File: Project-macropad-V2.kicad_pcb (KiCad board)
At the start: 2 copper layers, 110.5 x 128.4 mm, 51 parts, among them J1 Conn_01x04_Male, SW1 RotaryEncoder_Switch, SW2 SW_Push, SW3 SW_SPDT

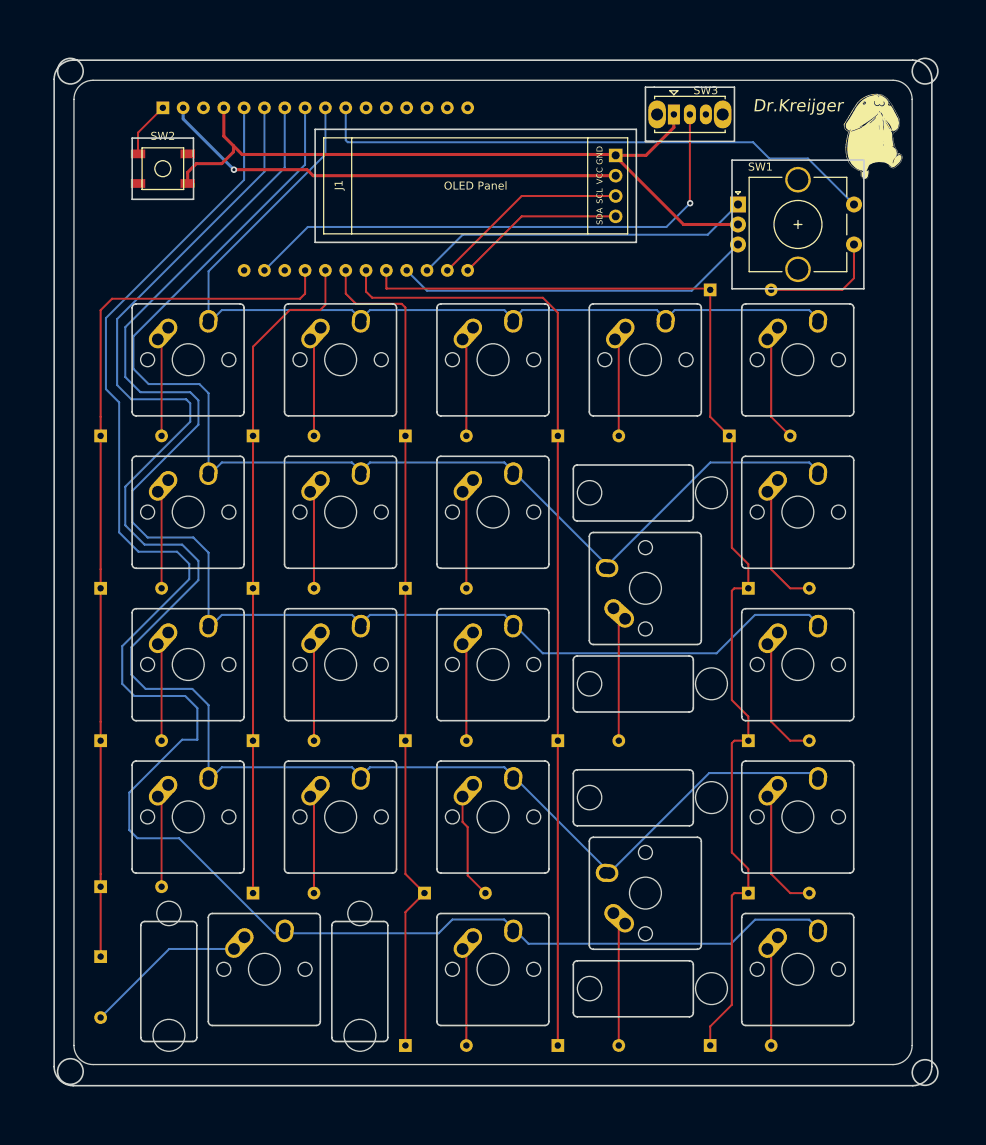
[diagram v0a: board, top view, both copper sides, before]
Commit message: Plate done
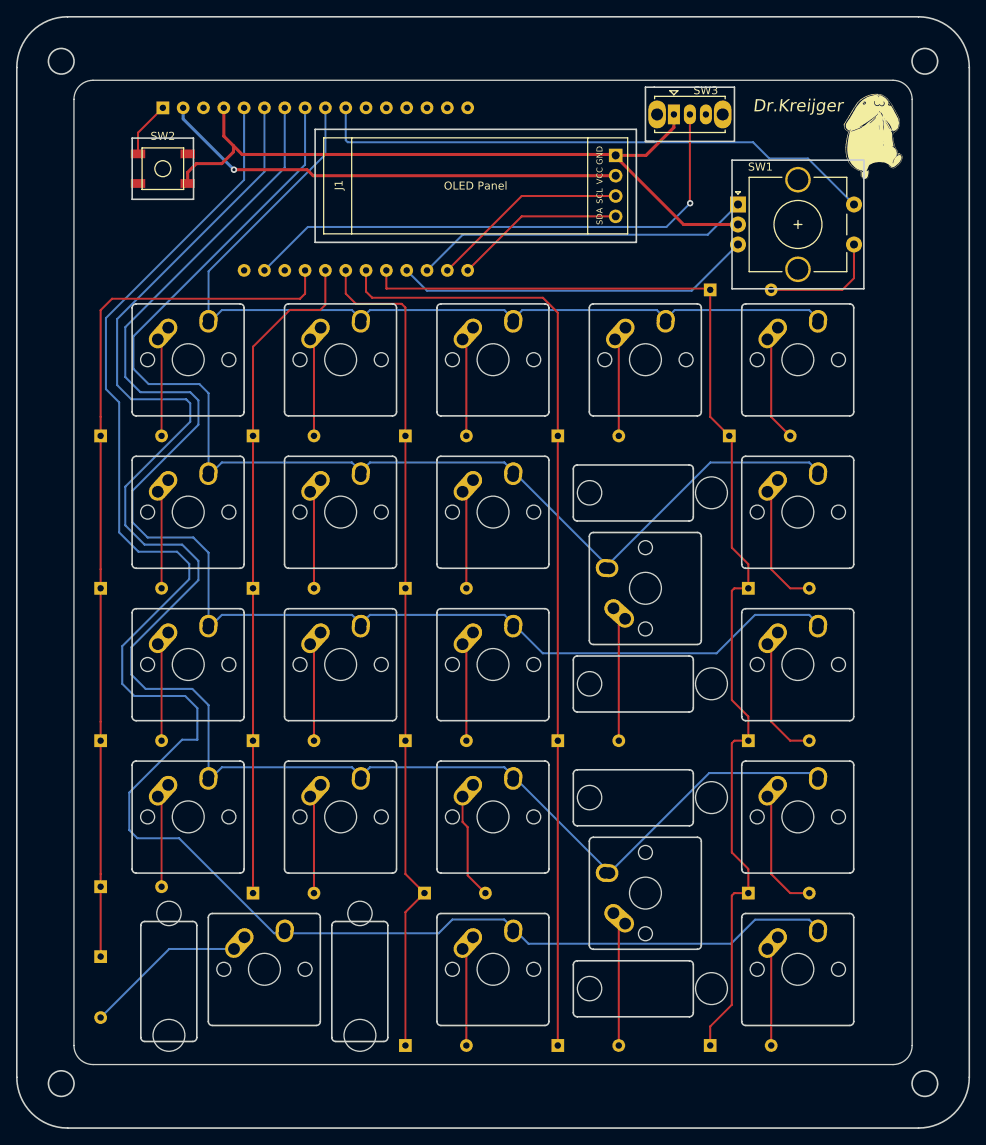
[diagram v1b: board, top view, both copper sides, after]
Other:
- board size 110.5 x 128.4 mm -> 119.1 x 138.9 mm
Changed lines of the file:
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@@
   (gr_line (start 113.635 50.673) (end 113.635 63.673) (layer "Edge.Cuts") (width 0.2))
   (gr_line (start 203.835 88.773) (end 203.835 101.773) (layer "Edge.Cuts") (width 0.2))
-  (gr_line (start 106.26725 147.898) (end 211.219002 147.898) (layer "Edge.Cuts") (width 0.2))
-  (gr_circle (center 105.918 21.082) (end 107.518 21.082) (layer "Edge.Cuts") (width 0.2) (fill none))
+  (gr_circle (center 104.775 19.84375) (end 106.375 19.84375) (layer "Edge.Cuts") (width 0.2) (fill none))
   (gr_arc (start 189.835 126.873) (mid 189.981447 126.519447) (end 190.335 126.373) (layer "Edge.Cuts") (width 0.2))
   (gr_arc (start 152.235 83.223) (mid 151.881447 83.076553) (end 151.735 82.723) (layer "Edge.Cuts") (width 0.2))
@@
   (gr_arc (start 127.135 88.273) (mid 127.488553 88.419447) (end 127.635 88.773) (layer "Edge.Cuts") (width 0.2))
   (gr_line (start 132.685 69.723) (end 132.685 82.723) (layer "Edge.Cuts") (width 0.2))
+  (gr_arc (start 211.93125 14.2875) (mid 216.421378 16.147372) (end 218.28125 20.6375) (layer "Edge.Cuts") (width 0.2))
   (gr_line (start 132.685 50.673) (end 132.685 63.673) (layer "Edge.Cuts") (width 0.2))
   (gr_line (start 132.685 107.823) (end 132.685 120.823) (layer "Edge.Cuts") (width 0.2))
   (gr_arc (start 170.785 79.248) (mid 170.931447 78.894447) (end 171.285 78.748) (layer "Edge.Cuts") (width 0.2))
+  (gr_line (start 99.21875 20.6375) (end 99.21875 146.84375) (layer "Edge.Cuts") (width 0.2))
   (gr_arc (start 113.635 107.823) (mid 113.781447 107.469447) (end 114.135 107.323) (layer "Edge.Cuts") (width 0.2))
   (gr_line (start 113.6396 29.448) (end 113.6396 37.084) (layer "Edge.Cuts") (width 0.2))
@@
   (gr_arc (start 127.635 63.673) (mid 127.488553 64.026553) (end 127.135 64.173) (layer "Edge.Cuts") (width 0.2))
   (gr_arc (start 123.16 126.873) (mid 123.306447 126.519447) (end 123.66 126.373) (layer "Edge.Cuts") (width 0.2))
-  (gr_circle (center 212.7506 21.082) (end 214.3506 21.082) (layer "Edge.Cuts") (width 0.2) (fill none))
+  (gr_circle (center 212.725 19.84375) (end 214.325 19.84375) (layer "Edge.Cuts") (width 0.2) (fill none))
   (gr_line (start 152.235 121.323) (end 165.235 121.323) (layer "Edge.Cuts") (width 0.2))
   (gr_arc (start 203.335 50.173) (mid 203.688553 50.319447) (end 203.835 50.673) (layer "Edge.Cuts") (width 0.2))
@@
   (gr_arc (start 127.135 50.173) (mid 127.488553 50.319447) (end 127.635 50.673) (layer "Edge.Cuts") (width 0.2))
   (gr_line (start 114.135 107.323) (end 127.135 107.323) (layer "Edge.Cuts") (width 0.2))
-  (gr_line (start 213.600252 145.51675) (end 213.600252 22.09165) (layer "Edge.Cuts") (width 0.2))
-  (gr_arc (start 213.600252 145.51675) (mid 212.9028 147.200548) (end 211.219002 147.898) (layer "Edge.Cuts") (width 0.2))
   (gr_line (start 170.785 79.248) (end 170.785 92.248) (layer "Edge.Cuts") (width 0.2))
   (gr_arc (start 189.835 50.673) (mid 189.981447 50.319447) (end 190.335 50.173) (layer "Edge.Cuts") (width 0.2))
@@
   (gr_line (start 170.785 50.673) (end 170.785 63.673) (layer "Edge.Cuts") (width 0.2))
   (gr_arc (start 183.285 108.41) (mid 183.638553 108.556447) (end 183.785 108.91) (layer "Edge.Cuts") (width 0.2))
-  (gr_line (start 211.219002 19.7104) (end 106.26725 19.7104) (layer "Edge.Cuts") (width 0.2))
   (gr_line (start 190.335 88.273) (end 203.335 88.273) (layer "Edge.Cuts") (width 0.2))
   (gr_line (start 151.735 50.673) (end 151.735 63.673) (layer "Edge.Cuts") (width 0.2))
@@
   (gr_arc (start 168.785 70.81) (mid 168.931447 70.456447) (end 169.285 70.31) (layer "Edge.Cuts") (width 0.2))
   (gr_arc (start 203.835 101.773) (mid 203.688553 102.126553) (end 203.335 102.273) (layer "Edge.Cuts") (width 0.2))
+  (gr_line (start 218.28125 146.84375) (end 218.28125 20.6375) (layer "Edge.Cuts") (width 0.2))
   (gr_line (start 190.335 50.173) (end 203.335 50.173) (layer "Edge.Cuts") (width 0.2))
   (gr_arc (start 165.235 88.273) (mid 165.588553 88.419447) (end 165.735 88.773) (layer "Edge.Cuts") (width 0.2))
@@
   (gr_line (start 208.75625 22.225) (end 108.74375 22.225) (layer "Edge.Cuts") (width 0.1))
   (gr_line (start 146.685 88.773) (end 146.685 101.773) (layer "Edge.Cuts") (width 0.2))
+  (gr_arc (start 105.56875 153.19375) (mid 101.078622 151.333878) (end 99.21875 146.84375) (layer "Edge.Cuts") (width 0.2))
   (gr_arc (start 203.335 69.223) (mid 203.688553 69.369447) (end 203.835 69.723) (layer "Edge.Cuts") (width 0.2))
   (gr_arc (start 208.75625 22.225) (mid 210.440048 22.922452) (end 211.1375 24.60625) (layer "Edge.Cuts") (width 0.1))
@@
   (gr_line (start 113.635 69.723) (end 113.635 82.723) (layer "Edge.Cuts") (width 0.2))
   (gr_arc (start 189.835 88.773) (mid 189.981447 88.419447) (end 190.335 88.273) (layer "Edge.Cuts") (width 0.2))
-  (gr_arc (start 211.219002 19.7104) (mid 212.9028 20.407852) (end 213.600252 22.09165) (layer "Edge.Cuts") (width 0.2))
   (gr_line (start 189.835 69.723) (end 189.835 82.723) (layer "Edge.Cuts") (width 0.2))
   (gr_arc (start 211.1375 142.875) (mid 210.440048 144.558798) (end 208.75625 145.25625) (layer "Edge.Cuts") (width 0.1))
   (gr_line (start 183.285 115.41) (end 169.285 115.41) (layer "Edge.Cuts") (width 0.2))
+  (gr_line (start 211.93125 14.2875) (end 105.56875 14.2875) (layer "Edge.Cuts") (width 0.2))
   (gr_line (start 114.135 50.173) (end 127.135 50.173) (layer "Edge.Cuts") (width 0.2))
+  (gr_arc (start 218.28125 146.84375) (mid 216.421378 151.333878) (end 211.93125 153.19375) (layer "Edge.Cuts") (width 0.2))
   (gr_line (start 152.235 64.173) (end 165.235 64.173) (layer "Edge.Cuts") (width 0.2))
   (gr_line (start 114.135 88.273) (end 127.135 88.273) (layer "Edge.Cuts") (width 0.2))
@@
   (gr_arc (start 113.635 69.723) (mid 113.781447 69.369447) (end 114.135 69.223) (layer "Edge.Cuts") (width 0.2))
   (gr_arc (start 146.685 63.673) (mid 146.538553 64.026553) (end 146.185 64.173) (layer "Edge.Cuts") (width 0.2))
-  (gr_line (start 103.886 145.51675) (end 103.886 22.09165) (layer "Edge.Cuts") (width 0.2))
   (gr_arc (start 190.335 140.373) (mid 189.981447 140.226553) (end 189.835 139.873) (layer "Edge.Cuts") (width 0.2))
   (gr_line (start 123.66 140.373) (end 136.66 140.373) (layer "Edge.Cuts") (width 0.2))
-  (gr_arc (start 103.886 22.09165) (mid 104.583452 20.407852) (end 106.26725 19.7104) (layer "Edge.Cuts") (width 0.2))
   (gr_arc (start 146.685 101.773) (mid 146.538553 102.126553) (end 146.185 102.273) (layer "Edge.Cuts") (width 0.2))
   (gr_arc (start 113.635 88.773) (mid 113.781447 88.419447) (end 114.135 88.273) (layer "Edge.Cuts") (width 0.2))
@@
   (gr_line (start 127.635 107.823) (end 127.635 120.823) (layer "Edge.Cuts") (width 0.2))
   (gr_line (start 168.785 94.686) (end 168.785 100.686) (layer "Edge.Cuts") (width 0.2))
-  (gr_circle (center 105.918 146.1262) (end 107.518 146.1262) (layer "Edge.Cuts") (width 0.2) (fill none))
+  (gr_circle (center 104.775 147.6375) (end 106.375 147.6375) (layer "Edge.Cuts") (width 0.2) (fill none))
   (gr_line (start 108.74375 145.25625) (end 208.75625 145.25625) (layer "Edge.Cuts") (width 0.1))
   (gr_arc (start 183.285 70.31) (mid 183.638553 70.456447) (end 183.785 70.81) (layer "Edge.Cuts") (width 0.2))
@@
   (gr_line (start 152.235 102.273) (end 165.235 102.273) (layer "Edge.Cuts") (width 0.2))
   (gr_line (start 168.785 70.81) (end 168.785 76.81) (layer "Edge.Cuts") (width 0.2))
+  (gr_line (start 105.56875 153.19375) (end 211.93125 153.19375) (layer "Edge.Cuts") (width 0.2))
   (gr_line (start 168.785 108.91) (end 168.785 114.91) (layer "Edge.Cuts") (width 0.2))
   (gr_line (start 113.635 88.773) (end 113.635 101.773) (layer "Edge.Cuts") (width 0.2))
@@
   (gr_arc (start 127.635 101.773) (mid 127.488553 102.126553) (end 127.135 102.273) (layer "Edge.Cuts") (width 0.2))
   (gr_arc (start 132.685 88.773) (mid 132.831447 88.419447) (end 133.185 88.273) (layer "Edge.Cuts") (width 0.2))
+  (gr_arc (start 99.21875 20.6375) (mid 101.078622 16.147372) (end 105.56875 14.2875) (layer "Edge.Cuts") (width 0.2))
   (gr_arc (start 190.335 83.223) (mid 189.981447 83.076553) (end 189.835 82.723) (layer "Edge.Cuts") (width 0.2))
   (gr_line (start 121.3104 37.1) (end 113.6396 37.1) (layer "Edge.Cuts") (width 0.2))
@@
   (gr_line (start 127.635 88.773) (end 127.635 101.773) (layer "Edge.Cuts") (width 0.2))
   (gr_line (start 152.235 50.173) (end 165.235 50.173) (layer "Edge.Cuts") (width 0.2))
-  (gr_arc (start 106.26725 147.898) (mid 104.583452 147.200548) (end 103.886 145.51675) (layer "Edge.Cuts") (width 0.2))
   (gr_arc (start 145.598 141.873) (mid 145.451553 142.226553) (end 145.098 142.373) (layer "Edge.Cuts") (width 0.2))
   (gr_arc (start 189.835 107.823) (mid 189.981447 107.469447) (end 190.335 107.323) (layer "Edge.Cuts") (width 0.2))
@@
   (gr_line (start 190.335 126.373) (end 203.335 126.373) (layer "Edge.Cuts") (width 0.2))
   (gr_arc (start 114.135 83.223) (mid 113.781447 83.076553) (end 113.635 82.723) (layer "Edge.Cuts") (width 0.2))
-  (gr_circle (center 212.7506 146.2532) (end 214.3506 146.2532) (layer "Edge.Cuts") (width 0.2) (fill none))
+  (gr_circle (center 212.725 147.6375) (end 214.325 147.6375) (layer "Edge.Cuts") (width 0.2) (fill none))
   (gr_arc (start 165.735 82.723) (mid 165.588553 83.076553) (end 165.235 83.223) (layer "Edge.Cuts") (width 0.2))
   (gr_line (start 133.185 69.223) (end 146.185 69.223) (layer "Edge.Cuts") (width 0.2))
